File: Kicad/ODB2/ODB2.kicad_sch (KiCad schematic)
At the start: 32 parts, among them U1 STM32F412ZGTx

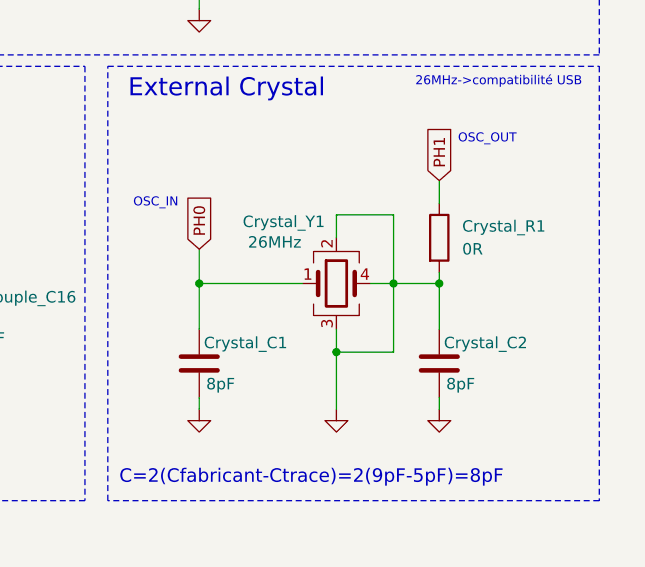
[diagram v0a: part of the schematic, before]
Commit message: Minor fix et début layout STM et sensors
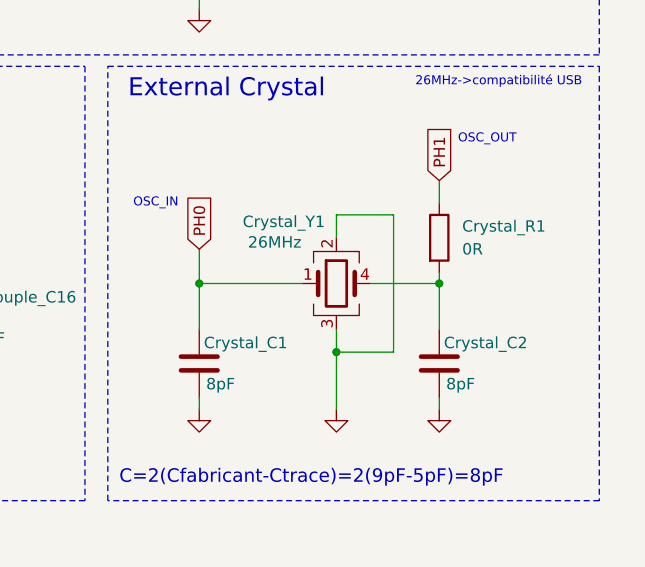
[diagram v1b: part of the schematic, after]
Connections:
- net GND: no longer Crystal_C2.1, Crystal_R1.2, Crystal_Y1.4
- new net: Crystal_C2.1, Crystal_R1.2, Crystal_Y1.4
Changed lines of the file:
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@@
-	)
-	(junction
-		(at 382.27 134.62)
-		(diameter 0)
-		(color 0 0 0 0)
 	)
 	(junction
@@
 	(wire
 		(pts
-			(xy 387.35 134.62) (xy 382.27 134.62)
-		)
-		(stroke
-			(width 0)
-			(type default)
-		)
-	)
-	(wire
-		(pts
 			(xy 165.1 160.02) (xy 170.18 160.02)
 		)
@@
 	(wire
 		(pts
-			(xy 382.27 127) (xy 382.27 134.62)
+			(xy 382.27 127) (xy 382.27 142.24)
 		)
 		(stroke
@@
 	(wire
 		(pts
-			(xy 379.73 134.62) (xy 382.27 134.62)
+			(xy 379.73 134.62) (xy 387.35 134.62)
 		)
 		(stroke
@@
 		)
 		(stroke
-			(width 0)
-			(type default)
-		)
-	)
-	(wire
-		(pts
-			(xy 382.27 134.62) (xy 382.27 142.24)
-		)
-		(stroke
